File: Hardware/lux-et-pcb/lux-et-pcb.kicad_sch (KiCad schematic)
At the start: 88 parts, among them J1 Conn_01x03_Socket, J2 Conn_01x03_Socket, J3 Conn_01x03_Socket, J4 USB_C_Receptacle_PowerOnly_6P, Q1 PMOS, Q2 PMOS, Q3 AO3400A, Q4 AO3400A, Q5 AO3400A, Q7 2N7002K, U1 XL1509-5V, U2 AP2112K-3.3, U3 ESP32-WROOM-32, U4 TP4056

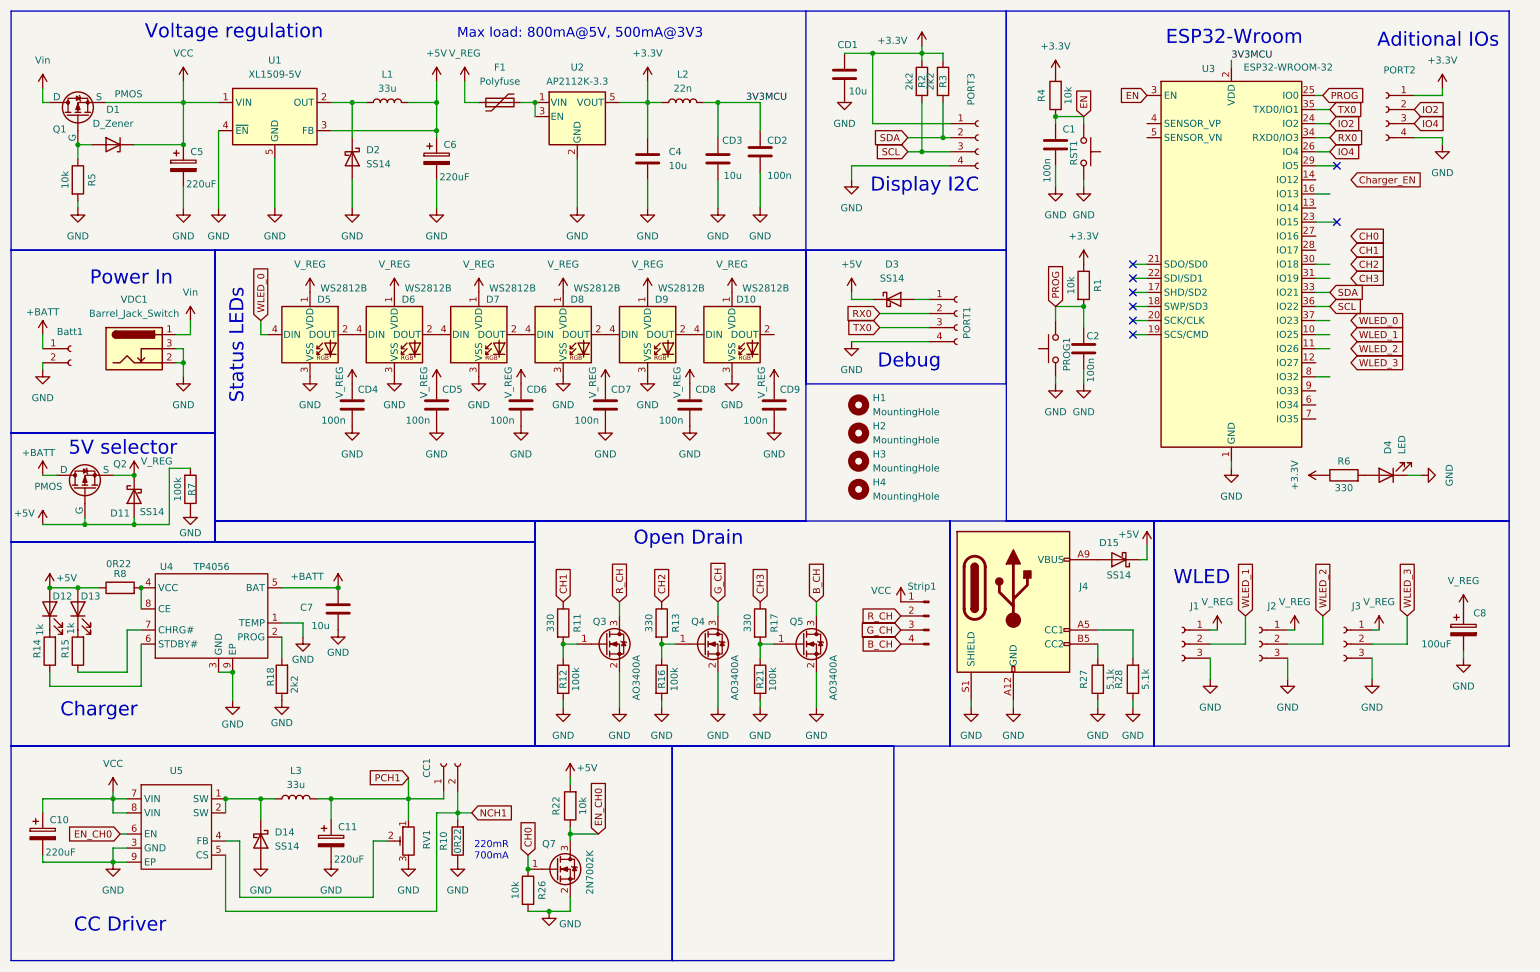
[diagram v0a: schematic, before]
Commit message: First finished layout for review
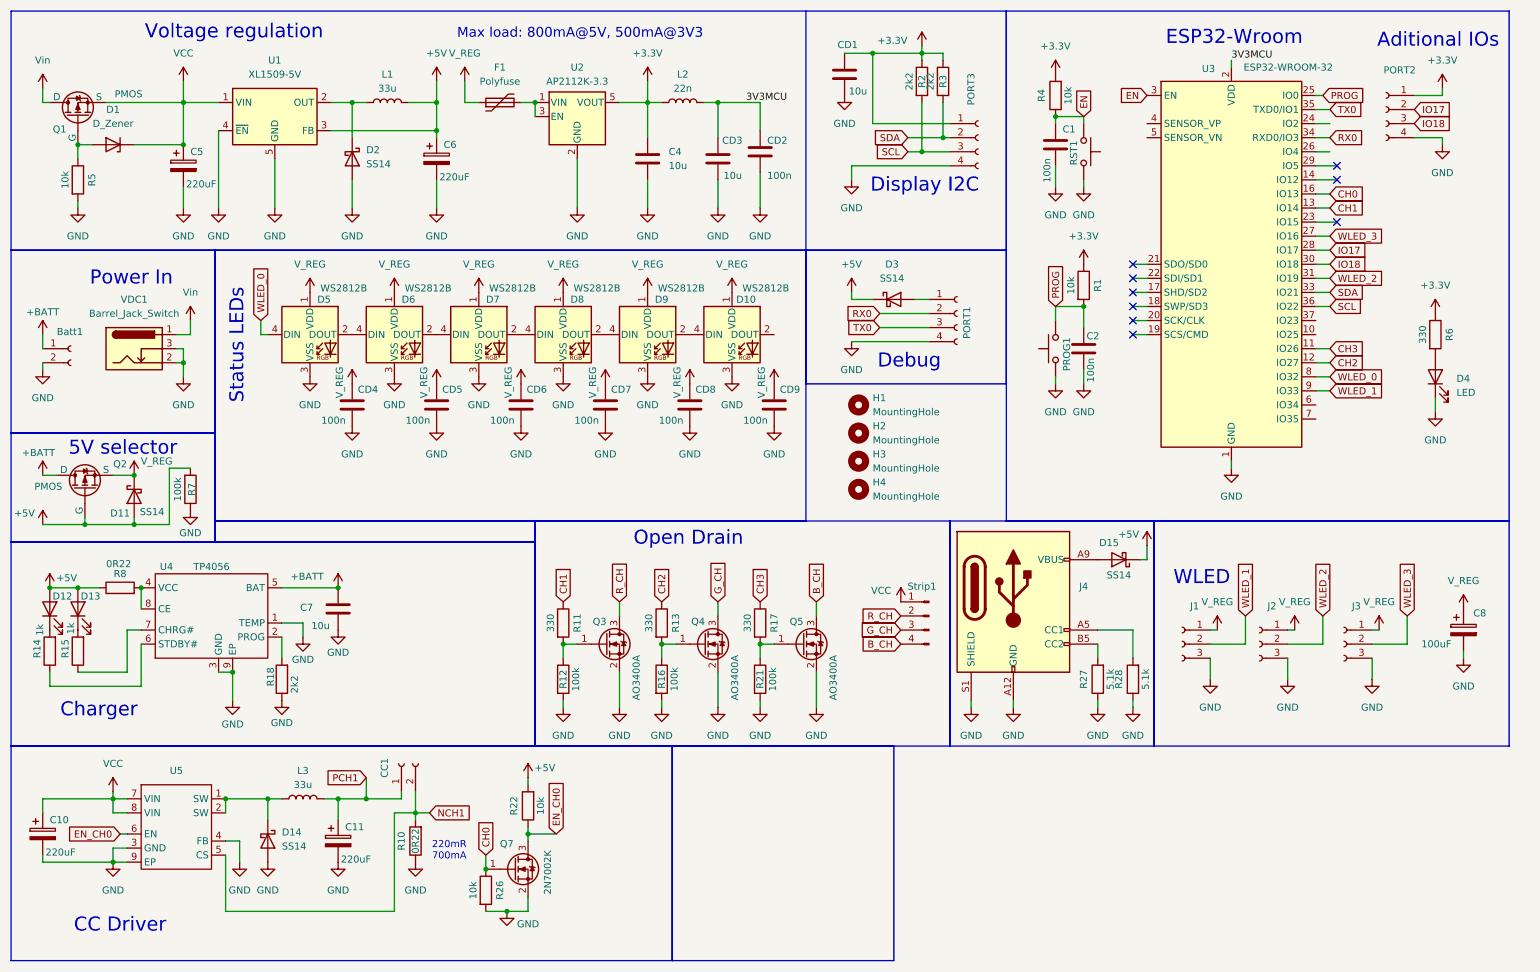
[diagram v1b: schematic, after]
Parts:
- removed RV1: R_Potentiometer_Trim, symbol Device:R_Potentiometer_Trim
- J4: footprint Connector_USB:USB_C_Receptacle_GCT_USB4125-xx-x-0190_6P_TopMnt_Horizontal -> Library:USB-C-SMD_GT-USB-7101A
- U3: footprint RF_Module:ESP32-WROOM-32 -> RF_Module:ESP32-WROOM-32U; symbol RF_Module:ESP32-WROOM-32 -> RF_Module:ESP32-WROOM-32U
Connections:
- net CH0: now also U3.16 (IO13)
- net CH1: now also U3.13 (IO14)
- net CH2: now also U3.12 (IO27)
- net CH3: now also U3.11 (IO26)
- net GND: now also U5.4 (FB)
- net WLED_0: now also U3.8 (IO32)
- net WLED_1: now also U3.9 (IO33)
- net WLED_2: now also U3.31 (IO19)
- net WLED_3: now also U3.27 (IO16)
- net IO17: now reaches U3.28 (IO17)
- net IO17: now also PORT2.2 (Pin_2)
- net IO18: now reaches U3.30 (IO18)
- net IO18: now also PORT2.3 (Pin_3)
- net IO2: no longer names the net of U3.24 (IO2)
- net IO2: no longer PORT2.2 (Pin_2)
- net IO4: no longer names the net of U3.26 (IO4)
- net IO4: no longer PORT2.3 (Pin_3)
- no-connect marks 8 -> 9
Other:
- moved on the sheet: C11, CC1, D14, D4, L3, Q7, R10, R22, R26, R6

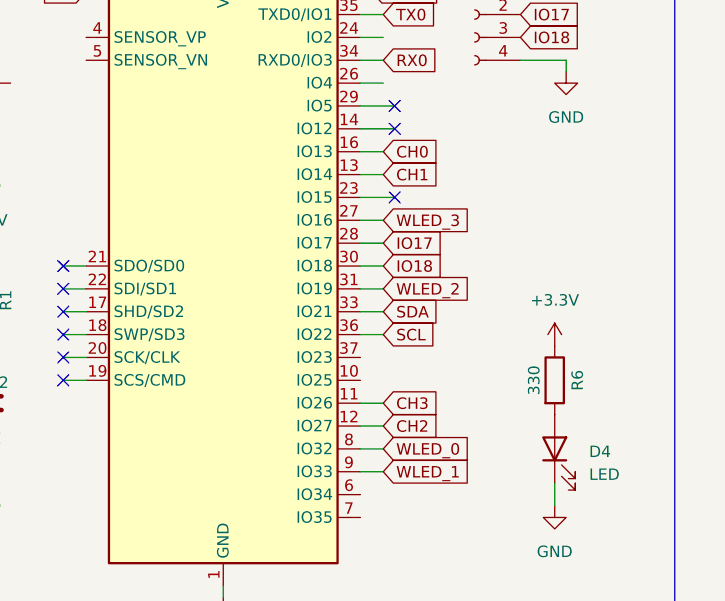
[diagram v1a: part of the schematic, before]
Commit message: Yet another version for review before fabrication
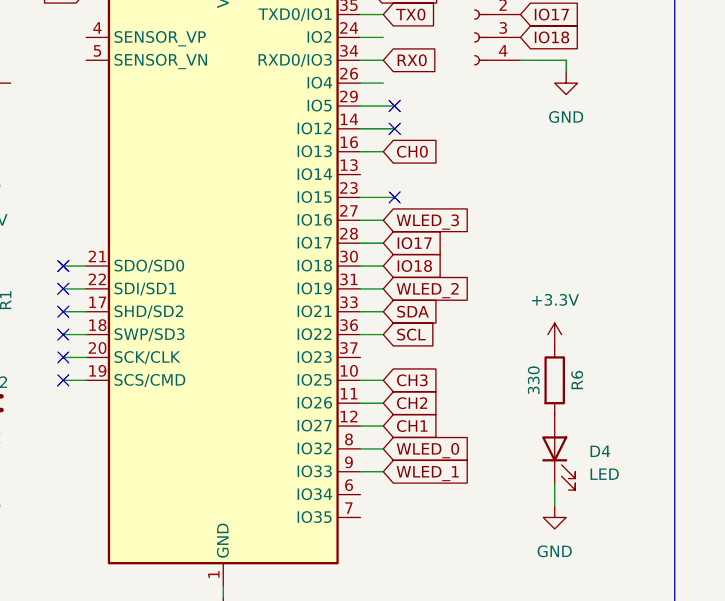
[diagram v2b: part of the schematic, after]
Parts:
- PORT1, PORT2: footprint Connector_Hirose:Hirose_DF13C_CL535-0404-8-51_1x04-1MP_P1.25mm_Vertical -> Library:Hirose_DF13C_CL535-0404-8-51_1x04-1MP_P1.25mm_Vertical
- PORT3: footprint Connector_Hirose:Hirose_DF13C_CL535-0404-8-51_1x04-1MP_P1.25mm_Vertical -> Library:Hirose_DF13C_CL535-0404-8-51_1x04-1MP_P1.25mm_Vertical; symbol Connector:Conn_01x04_Socket -> New_Library:Conn_01x04_Socket
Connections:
- net CH1: now also U3.12 (IO27); no longer U3.13 (IO14)
- net CH2: now also U3.11 (IO26); no longer U3.12 (IO27)
- net CH3: now also U3.10 (IO25); no longer U3.11 (IO26)
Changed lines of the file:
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@@
 	(wire
 		(pts
-			(xy 251.46 74.93) (xy 248.92 74.93)
-		)
-		(stroke
-			(width 0)
-			(type default)
-		)
-	)
-	(wire
-		(pts
 			(xy 130.81 128.27) (xy 130.81 130.81)
 		)
@@
 	(wire
 		(pts
-			(xy 251.46 49.53) (xy 248.92 49.53)
-		)
-		(stroke
-			(width 0)
-			(type default)
-		)
-	)
-	(wire
-		(pts
 			(xy 207.01 67.31) (xy 207.01 71.12)
 		)
@@
 	(wire
 		(pts
-			(xy 251.46 77.47) (xy 248.92 77.47)
+			(xy 248.92 72.39) (xy 251.46 72.39)
 		)
 		(stroke
@@
 	(wire
 		(pts
+			(xy 248.92 74.93) (xy 251.46 74.93)
+		)
+		(stroke
+			(width 0)
+			(type default)
+		)
+	)
+	(wire
+		(pts
 			(xy 25.4 133.35) (xy 34.29 133.35)
 		)
@@
 	(wire
 		(pts
+			(xy 248.92 77.47) (xy 251.46 77.47)
+		)
+		(stroke
+			(width 0)
+			(type default)
+		)
+	)
+	(wire
+		(pts
 			(xy 90.17 44.45) (xy 90.17 49.53)
 		)
@@
 	(global_label "CH1"
 		(shape input)
-		(at 251.46 49.53 0)
+		(at 251.46 77.47 0)
 		(fields_autoplaced yes)
 		(effects
@@
 		)
 		(property "Intersheetrefs" "${INTERSHEET_REFS}"
-			(at 258.2552 49.53 0)
+			(at 258.2552 77.47 0)
 			(effects
 				(font
@@
 	(global_label "CH2"
 		(shape input)
-		(at 251.46 77.47 0)
+		(at 251.46 74.93 0)
 		(fields_autoplaced yes)
 		(effects
@@
 		)
 		(property "Intersheetrefs" "${INTERSHEET_REFS}"
-			(at 258.2552 77.47 0)
+			(at 258.2552 74.93 0)
 			(effects
 				(font
@@
 	(global_label "CH3"
 		(shape input)
-		(at 251.46 74.93 0)
+		(at 251.46 72.39 0)
 		(fields_autoplaced yes)
 		(effects
@@
 		)
 		(property "Intersheetrefs" "${INTERSHEET_REFS}"
-			(at 258.2552 74.93 0)
+			(at 258.2552 72.39 0)
 			(effects
 				(font
@@
 			)
 		)
-		(property "Footprint" "Connector_Hirose:Hirose_DF13C_CL535-0404-8-51_1x04-1MP_P1.25mm_Vertical"
+		(property "Footprint" "Library:Hirose_DF13C_CL535-0404-8-51_1x04-1MP_P1.25mm_Vertical"
 			(at 261.62 31.75 0)
 			(effects
@@
 			)
 		)
-		(property "Footprint" "Connector_Hirose:Hirose_DF13C_CL535-0404-8-51_1x04-1MP_P1.25mm_Vertical"
+		(property "Footprint" "Library:Hirose_DF13C_CL535-0404-8-51_1x04-1MP_P1.25mm_Vertical"
 			(at 184.15 68.58 0)
 			(effects
@@
 	)
 	(symbol
-		(lib_id "Connector:Conn_01x04_Socket")
+		(lib_id "New_Library:Conn_01x04_Socket")
 		(at 187.96 36.83 0)
 		(unit 1)
@@
 			)
 		)
-		(property "Footprint" "Connector_Hirose:Hirose_DF13C_CL535-0404-8-51_1x04-1MP_P1.25mm_Vertical"
+		(property "Footprint" "Library:Hirose_DF13C_CL535-0404-8-51_1x04-1MP_P1.25mm_Vertical"
 			(at 187.96 36.83 0)
 			(effects
